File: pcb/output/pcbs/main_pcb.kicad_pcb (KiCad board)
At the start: 2 copper layers, 134.9 x 105.6 mm, 39 parts

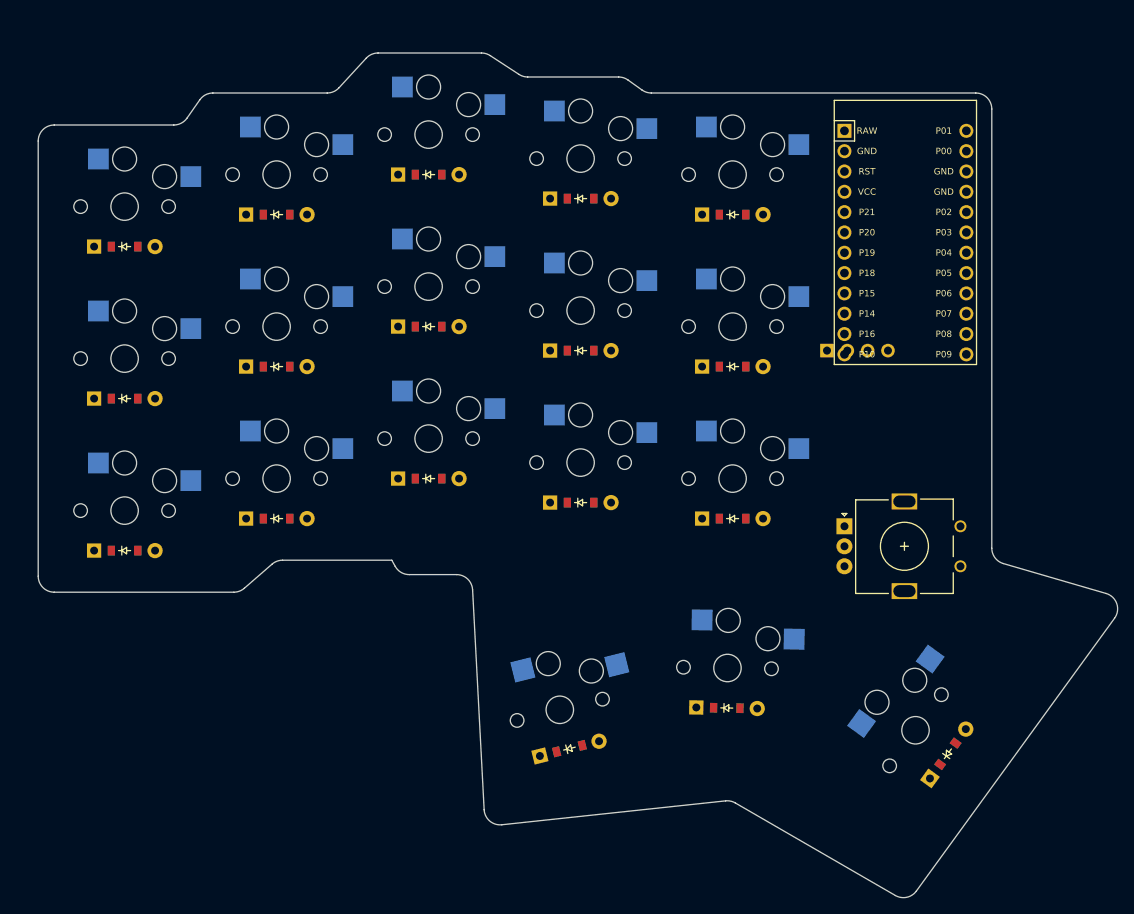
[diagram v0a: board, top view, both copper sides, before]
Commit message: pcb ready for order
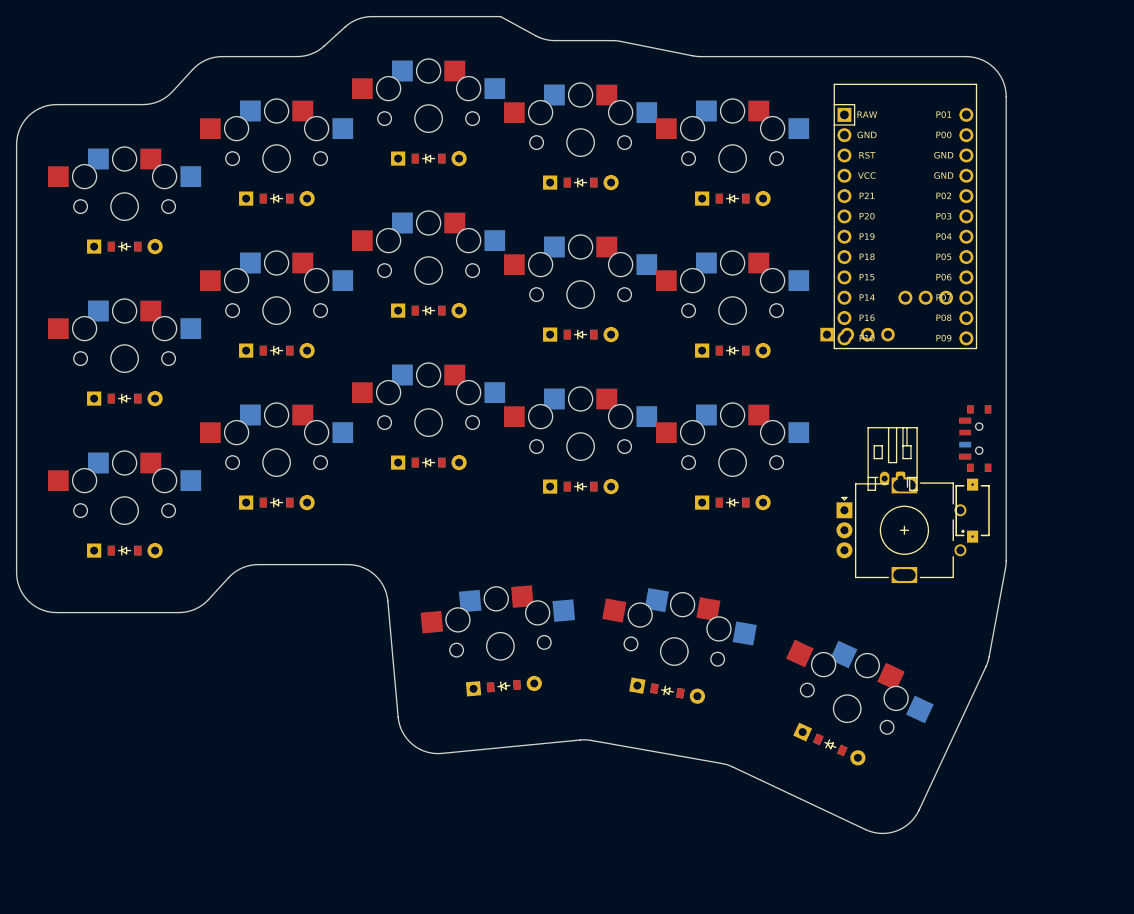
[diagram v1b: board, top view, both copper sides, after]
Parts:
- added S19: , 434121025816, F.Cu at (206.0, 100.0)
- added T1: , Button_Switch_SMD:SW_SPDT_PCM12, F.Cu at (206.5, 91.0)
- added _1: , Connector_JST:JST_PH_S2B-PH-K_1x02_P2.00mm_Horizontal,  at (197.0, 96.0)
- moved D18 14.7 mm to (188.2, 129.3), turned to -25 degrees
- moved D16 11.3 mm to (147.4, 121.9), turned to 5 degrees
- moved S16 10.9 mm to (147.0, 117.0), turned to 5 degrees
- moved S18 8.95 mm to (190.3, 124.8), turned to -25 degrees
- moved D17 7.72 mm to (167.8, 122.5), turned to -10 degrees
- moved S17 6.95 mm to (168.7, 117.6), turned to -10 degrees
- moved D10 2.00 mm to (157.0, 97.0)
- moved D11 2.00 mm to (157.0, 78.0)
- moved D12 2.00 mm to (157.0, 59.0)
- moved D13 2.00 mm to (176.0, 99.0)
- moved D14 2.00 mm to (176.0, 80.0)
- moved D15 2.00 mm to (176.0, 61.0)
- moved D4 2.00 mm to (119.0, 99.0)
- moved D5 2.00 mm to (119.0, 80.0)
- moved D6 2.00 mm to (119.0, 61.0)
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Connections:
- D1 pad 1: (no net) -> P19
- D10 pad 1: (no net) -> P19
- D11 pad 1: (no net) -> P20
- D12 pad 1: (no net) -> P21
- D13 pad 1: (no net) -> P19
- D14 pad 1: (no net) -> P20
- D15 pad 1: (no net) -> P21
- D16 pad 1: (no net) -> P18
- D17 pad 1: (no net) -> P18
- D18 pad 1: (no net) -> P18
- D2 pad 1: (no net) -> P20
- D3 pad 1: (no net) -> P21
- D4 pad 1: (no net) -> P19
- D5 pad 1: (no net) -> P20
- D6 pad 1: (no net) -> P21
- D7 pad 1: (no net) -> P19
- D8 pad 1: (no net) -> P20
- D9 pad 1: (no net) -> P21
- ROT1 pad 1: D7 -> NN_101
- ROT1 pad 2: E6 -> GND
- ROT1 pad A: B4 -> NN_102
- ROT1 pad B: B5 -> NN_107
- S1 pad 1: P14 -> P9
- S10 pad 1: P7 -> P6
- S11 pad 1: P7 -> P6
- S12 pad 1: P7 -> P6
- S13 pad 1: P9 -> P5
- S14 pad 1: P9 -> P5
- S15 pad 1: P9 -> P5
- S16 pad 1: (no net) -> P7
- S17 pad 1: (no net) -> P6
- S18 pad 1: (no net) -> P5
- S2 pad 1: P14 -> P9
- S3 pad 1: P14 -> P9
- S4 pad 1: P16 -> P8
- S5 pad 1: P16 -> P8
- S6 pad 1: P16 -> P8
- S7 pad 1: P10 -> P7
- S8 pad 1: P10 -> P7
- S9 pad 1: P10 -> P7
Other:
- board size 134.9 x 105.6 mm -> 123.7 x 102.1 mm
